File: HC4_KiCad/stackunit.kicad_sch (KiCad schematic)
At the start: 18 parts, among them IC11 74HC161, IC12 74HC377

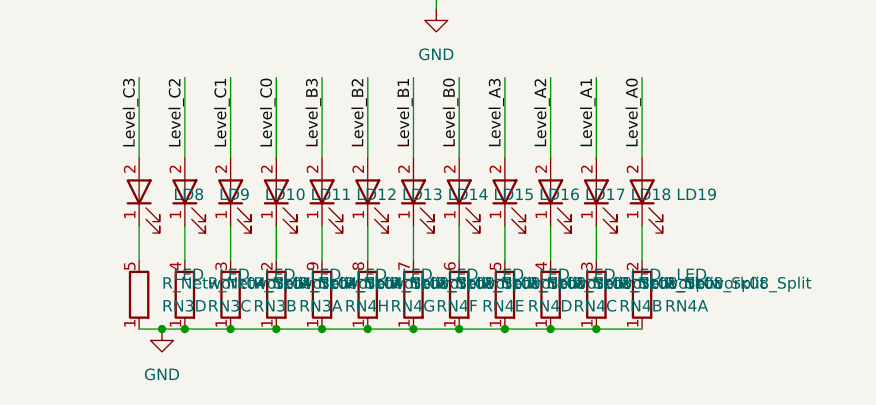
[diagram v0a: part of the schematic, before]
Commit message: ドキュメンテーションをちょっと充実
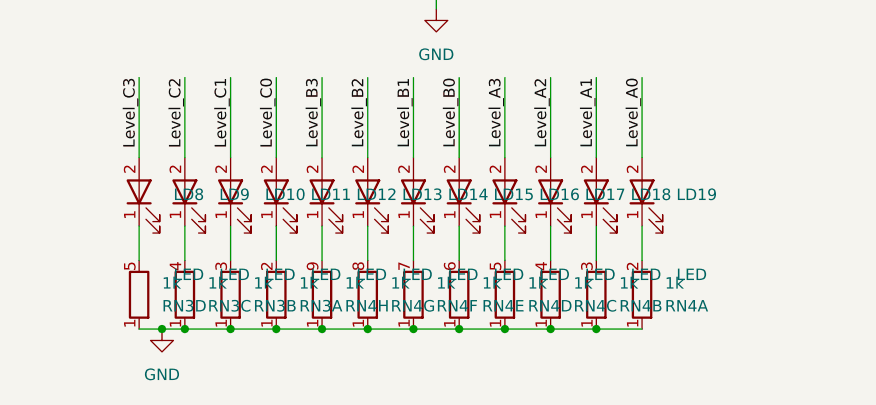
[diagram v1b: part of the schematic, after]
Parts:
- RN3: value R_Network04_Split -> 1k
- RN4: value R_Network08_Split -> 1k
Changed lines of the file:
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@@
 			)
 		)
-		(property "Value" "R_Network04_Split"
+		(property "Value" "1k"
 			(at 147.32 153.6701 0)
 			(effects
@@
 			)
 		)
-		(property "Value" "R_Network04_Split"
+		(property "Value" "1k"
 			(at 152.4 153.6701 0)
 			(effects
@@
 			)
 		)
-		(property "Value" "R_Network08_Split"
+		(property "Value" "1k"
 			(at 193.04 153.6701 0)
 			(effects
@@
 			)
 		)
-		(property "Value" "R_Network08_Split"
+		(property "Value" "1k"
 			(at 187.96 153.6701 0)
 			(effects
@@
 			)
 		)
-		(property "Value" "R_Network08_Split"
+		(property "Value" "1k"
 			(at 157.48 153.6701 0)
 			(effects
@@
 			)
 		)
-		(property "Value" "R_Network04_Split"
+		(property "Value" "1k"
 			(at 137.16 153.6701 0)
 			(effects
@@
 			)
 		)
-		(property "Value" "R_Network08_Split"
+		(property "Value" "1k"
 			(at 162.56 153.6701 0)
 			(effects
@@
 			)
 		)
-		(property "Value" "R_Network08_Split"
+		(property "Value" "1k"
 			(at 182.88 153.6701 0)
 			(effects
@@
 			)
 		)
-		(property "Value" "R_Network04_Split"
+		(property "Value" "1k"
 			(at 142.24 153.6701 0)
 			(effects
@@
 			)
 		)
-		(property "Value" "R_Network08_Split"
+		(property "Value" "1k"
 			(at 172.72 153.6701 0)
 			(effects
@@
 			)
 		)
-		(property "Value" "R_Network08_Split"
+		(property "Value" "1k"
 			(at 177.8 153.6701 0)
 			(effects
@@
 			)
 		)
-		(property "Value" "R_Network08_Split"
+		(property "Value" "1k"
 			(at 167.64 153.6701 0)
 			(effects
